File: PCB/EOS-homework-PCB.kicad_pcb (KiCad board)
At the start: 4 copper layers, 30 parts, among them J2 Conn_ST_STDC14, J3 USB-C MCU, U1 STM32WB55CEU6, U2 MIC5365-3.3YD5, U7 USBLC6-2SC6

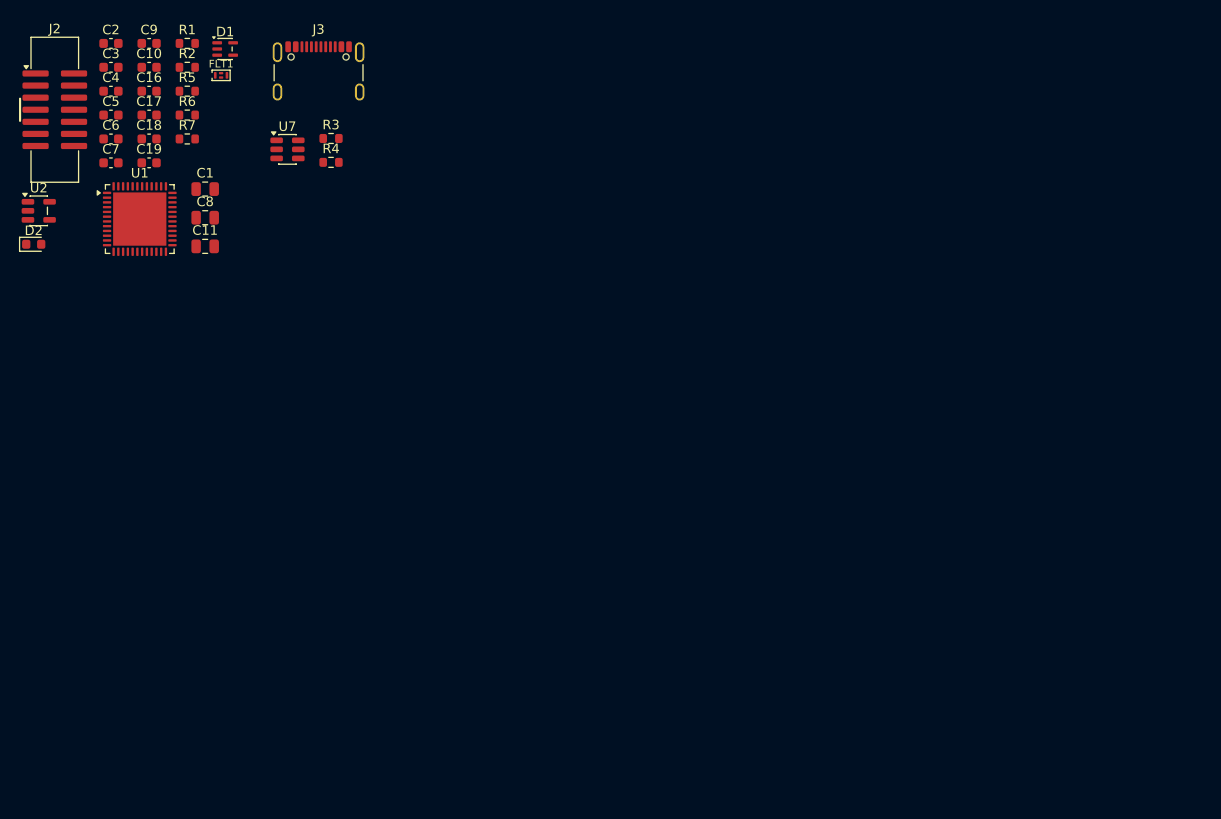
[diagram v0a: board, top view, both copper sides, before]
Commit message: PCB done.
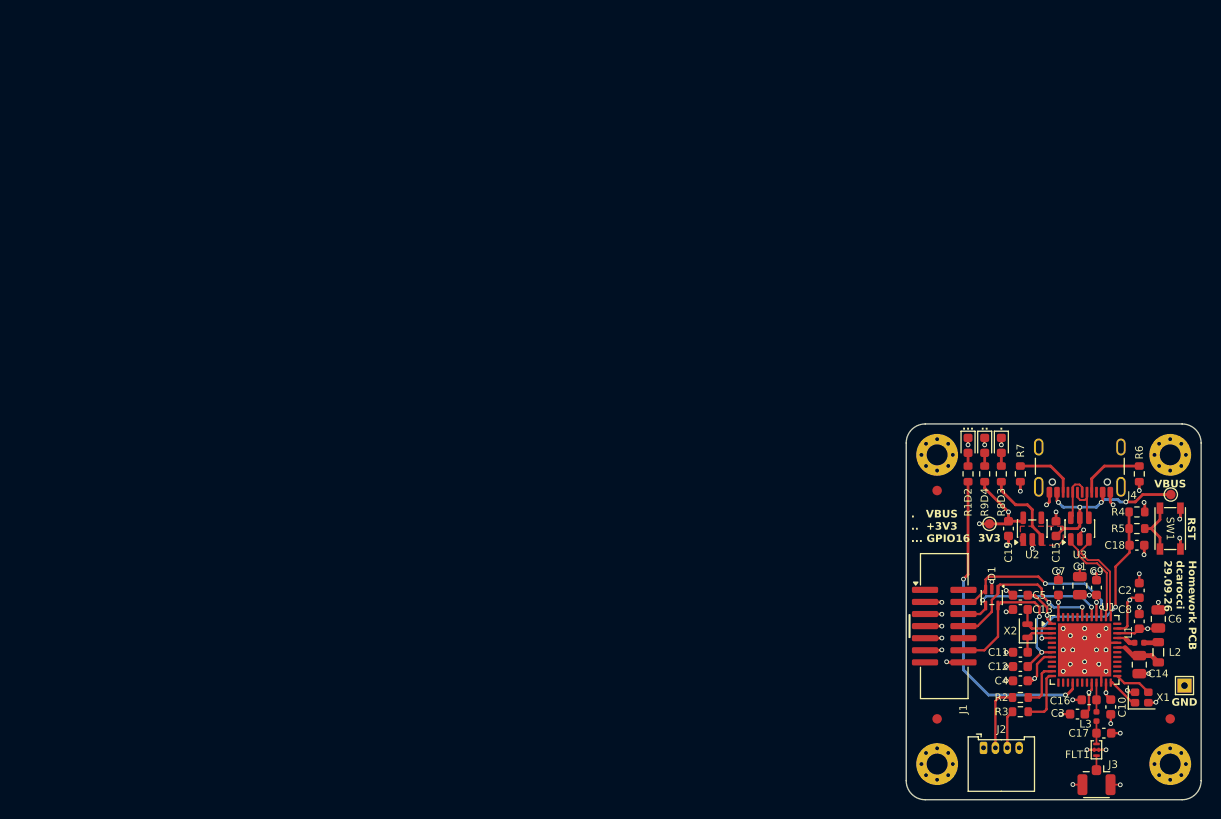
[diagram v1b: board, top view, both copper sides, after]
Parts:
- removed U7: USBLC6-2SC6, Package_TO_SOT_SMD:SOT-23-6
- added C12: 100n/50V, Capacitor_SMD:C_0603_1608Metric, F.Cu at (143.2, 103.5)
- added C13: 10p, Capacitor_SMD:C_0603_1608Metric, F.Cu at (143.2, 97.5)
- added C14: 4u7/16V, Capacitor_SMD:C_0805_2012Metric, F.Cu at (155.8, 103.3)
- added C15: 1u/50V, Capacitor_SMD:C_0603_1608Metric, F.Cu at (147.0, 89.0)
- added D3: Red, LED_SMD:LED_0603_1608Metric, F.Cu at (141.2, 80.2)
- added D4: Red, LED_SMD:LED_0603_1608Metric, F.Cu at (139.5, 80.2)
- added FID1: Fiducial, Fiducial:Fiducial_1mm_Mask2mm, F.Cu at (134.5, 85.0)
- added FID2: Fiducial, Fiducial:Fiducial_1mm_Mask2mm, F.Cu at (134.5, 109.0)
- added FID3: Fiducial, Fiducial:Fiducial_1mm_Mask2mm, F.Cu at (159.0, 109.0)
- added H1: MountingHole_Pad, MountingHole:MountingHole_2.2mm_M2_Pad_Via, F.Cu at (134.5, 81.2)
- added H2: MountingHole_Pad, MountingHole:MountingHole_2.2mm_M2_Pad_Via, F.Cu at (159.0, 81.2)
- added H3: MountingHole_Pad, MountingHole:MountingHole_2.2mm_M2_Pad_Via, F.Cu at (159.0, 113.8)
- added H4: MountingHole_Pad, MountingHole:MountingHole_2.2mm_M2_Pad_Via, F.Cu at (134.5, 113.8)
- added J1: Conn_ST_STDC14, kicad-standard-lib:IDC-Header_2x07_P1.27mm_Vertical_SMD, F.Cu at (135.2, 99.2)
- added J4: USB-C MCU, Connector_USB:USB_C_Receptacle_GCT_USB4105-xx-A_16P_TopMnt_Horizontal, F.Cu at (149.5, 81.5)
- added L1: 10n, Inductor_SMD:L_0402_1005Metric, F.Cu at (155.8, 101.0)
- added L2: 10u, Inductor_SMD:L_0805_2012Metric, F.Cu at (157.8, 102.0)
- added L3: 2n7, Inductor_SMD:L_0402_1005Metric, F.Cu at (151.2, 108.8)
- added R8: 1k, Resistor_SMD:R_0603_1608Metric, F.Cu at (141.2, 83.2)
- added R9: 1k, Resistor_SMD:R_0603_1608Metric, F.Cu at (139.5, 83.2)
- added SW1: Reset, kicad-standard-lib:SW_Push_Wuerth_434123025826, F.Cu at (159.0, 89.0)
- added TP1: TestPoint, TestPoint:TestPoint_Pad_D1.0mm, F.Cu at (159.1, 85.4)
- added TP2: TestPoint, TestPoint:TestPoint_Pad_D1.0mm, F.Cu at (140.0, 88.5)
- added TP3: TestPoint_Square, TestPoint:TestPoint_THTPad_1.5x1.5mm_Drill0.7mm, F.Cu at (160.5, 105.5)
- added U3: USBLC6-2SC6, Package_TO_SOT_SMD:SOT-23-6, F.Cu at (149.5, 89.0)
- added X1: 32MHz, Crystal:Crystal_SMD_2016-4Pin_2.0x1.6mm, F.Cu at (156.0, 106.8)
- added X2: 32kHz768, Crystal:Crystal_SMD_2012-2Pin_2.0x1.2mm, F.Cu at (144.0, 99.8)
- C11: value 4u7/16V -> 10p; footprint Capacitor_SMD:C_0805_2012Metric -> Capacitor_SMD:C_0603_1608Metric
- C16: value 100n/50V -> 0p8
- C17: value 100n/50V -> 0p3
- C18: value 1u/50V -> 100n/50V
- C6: value 100n/50V -> 4u7/16V; footprint Capacitor_SMD:C_0603_1608Metric -> Capacitor_SMD:C_0805_2012Metric
- C8: value 4u7/16V -> 100n/50V; footprint Capacitor_SMD:C_0805_2012Metric -> Capacitor_SMD:C_0603_1608Metric
- J2: value Conn_ST_STDC14 -> Conn_01x04; footprint kicad-standard-lib:IDC-Header_2x07_P1.27mm_Vertical_SMD -> Connector_Molex:Molex_PicoBlade_53048-0410_1x04_P1.25mm_Horizontal
- J3: value USB-C MCU -> Conn_Coaxial; footprint Connector_USB:USB_C_Receptacle_GCT_USB4105-xx-A_16P_TopMnt_Horizontal -> Connector_Coaxial:U.FL_Hirose_U.FL-R-SMT-1_Vertical
- R1: value 10k -> 1k
- R3: value 5k1 -> 100R
- R4: value 5k1 -> 10k
- R6: value 100R -> 5k1
- R7: value 1k -> 5k1
- moved C2 122.4 mm to (155.8, 95.5), turned to 90 degrees
- moved C3 122.2 mm to (149.2, 108.5), turned to 180 degrees
- moved C10 121.4 mm to (152.8, 107.8), turned to -90 degrees
- moved C6 121.1 mm to (157.8, 98.5), turned to 90 degrees
- moved C17 119.5 mm to (152.0, 110.5)
- moved J2 118.4 mm to (139.4, 112.0)
- moved C16 117.7 mm to (150.5, 107.0), turned to 180 degrees
- moved FLT1 116.2 mm to (151.2, 112.2), turned to -90 degrees
- moved C9 114.8 mm to (151.2, 95.2), turned to 90 degrees
- moved C4 113.9 mm to (143.2, 105.0), turned to 180 degrees
- moved C18 112.3 mm to (155.5, 90.8)
- moved J3 110.2 mm to (151.2, 115.9), turned to -90 degrees
- moved R5 109.9 mm to (155.5, 89.0)
- moved R2 109.8 mm to (143.2, 106.8)
- moved U2 109.6 mm to (144.5, 89.0), turned to 90 degrees
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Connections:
- C11 pad 1: /Microcontroller/SMPSFB -> /Microcontroller/LSE_OUT
- C16 pad 1: /Microcontroller/~{Reset} -> /Microcontroller/RF
- C17 pad 1: /Microcontroller/BOOT0 -> /Microcontroller/RF_MATCH
- C18 pad 1: +5V -> /Microcontroller/BOOT0
- D1 pad 5: /Microcontroller/~{Reset} -> /Microcontroller/SW_~{Reset}
- D2 pad 1: Net-(D2-K) -> GND
- D2 pad 2: /Microcontroller/LED -> Net-(D2-A)
- J2 pad 1: unconnected-(J2-NC-Pad1) -> +3.3V
- J2 pad 2: unconnected-(J2-NC-Pad2) -> /Microcontroller/UART_TXC
- J2 pad 3: +5V -> /Microcontroller/UART_RXC
- J2 pad 4: /Microcontroller/SWDIO -> GND
- R1 pad 1: /Microcontroller/BOOT0 -> Net-(D2-A)
- R1 pad 2: GND -> /Microcontroller/LED
- R2 pad 1: /Microcontroller/BOOT0 -> /Microcontroller/UART_TXC
- R2 pad 2: Net-(R2-Pad2) -> /Microcontroller/UART_TX
- R3 pad 1: GND -> /Microcontroller/UART_RX
- R3 pad 2: Net-(J3-CC1) -> /Microcontroller/UART_RXC
- R4 pad 1: GND -> /Microcontroller/BOOT0
- R4 pad 2: Net-(J3-CC2) -> GND
- R5 pad 1: /Microcontroller/UART_TXC -> /Microcontroller/BOOT0
- R5 pad 2: /Microcontroller/UART_TX -> Net-(R5-Pad2)
- R6 pad 1: /Microcontroller/UART_RX -> GND
- R6 pad 2: /Microcontroller/UART_RXC -> Net-(J4-CC1)
- R7 pad 2: Net-(D2-K) -> Net-(J4-CC2)
- U1 pad 7: /Microcontroller/~{Reset} -> /Microcontroller/SW_~{Reset}
- U2 pad 1: +5V -> VBUS
- U2 pad 3: +5V -> VBUS
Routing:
- net GND: track 0.00 -> 50.9 mm, vias 0 -> 57
- net +3.3V: track 0.00 -> 44.9 mm, vias 0 -> 14
- net /Microcontroller/LED: track 0.00 -> 33.5 mm, vias 0 -> 2
- net VBUS: track 0.00 -> 28.6 mm, vias 0 -> 4
- net /Microcontroller/BOOT0: track 0.00 -> 21.4 mm, vias 0 -> 2
- net /Microcontroller/SW_~{Reset}: track 0.00 -> 20.4 mm, vias 0 -> 2
- net /Microcontroller/SWDIO: track 0.00 -> 19.1 mm, vias 0 -> 2
- net /Microcontroller/SWO: track 0.00 -> 17.9 mm, vias 0 -> 2
- net /Microcontroller/SWCLK: track 0.00 -> 16.8 mm, vias 0 -> 2
- net /Microcontroller/USB_D-: track 0.00 -> 10.4 mm
- net /Microcontroller/USB_D+: track 0.00 -> 10.4 mm
- net Net-(J4-CC1): track 0.00 -> 6.98 mm
- net /Microcontroller/UART_TXC: track 0.00 -> 6.88 mm
- net Net-(J4-CC2): track 0.00 -> 6.48 mm
- net /Microcontroller/UART_RX: track 0.00 -> 5.94 mm
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- added copper zone on In2.Cu, net +3.3V
- added copper zone on In1.Cu, net GND
- added copper zone on F.Cu, net VBUS
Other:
- board outline added: 31 x 39.5 mm
- board text added: "."
- board text added: ". VBUS .. +3V3 ... GPIO16"
- board text added: ".."
- board text added: "..."
- board text added: "3V3"
- board text added: "GND"
- board text added: "Homework PCB dcarocci 29.09.26"
- board text added: "RST"
- board text added: "VBUS"
